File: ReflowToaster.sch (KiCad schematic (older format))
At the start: 3 parts, among them J2 USB-Micro-B, J3 USB-Micro-B, Q1 FDN340P

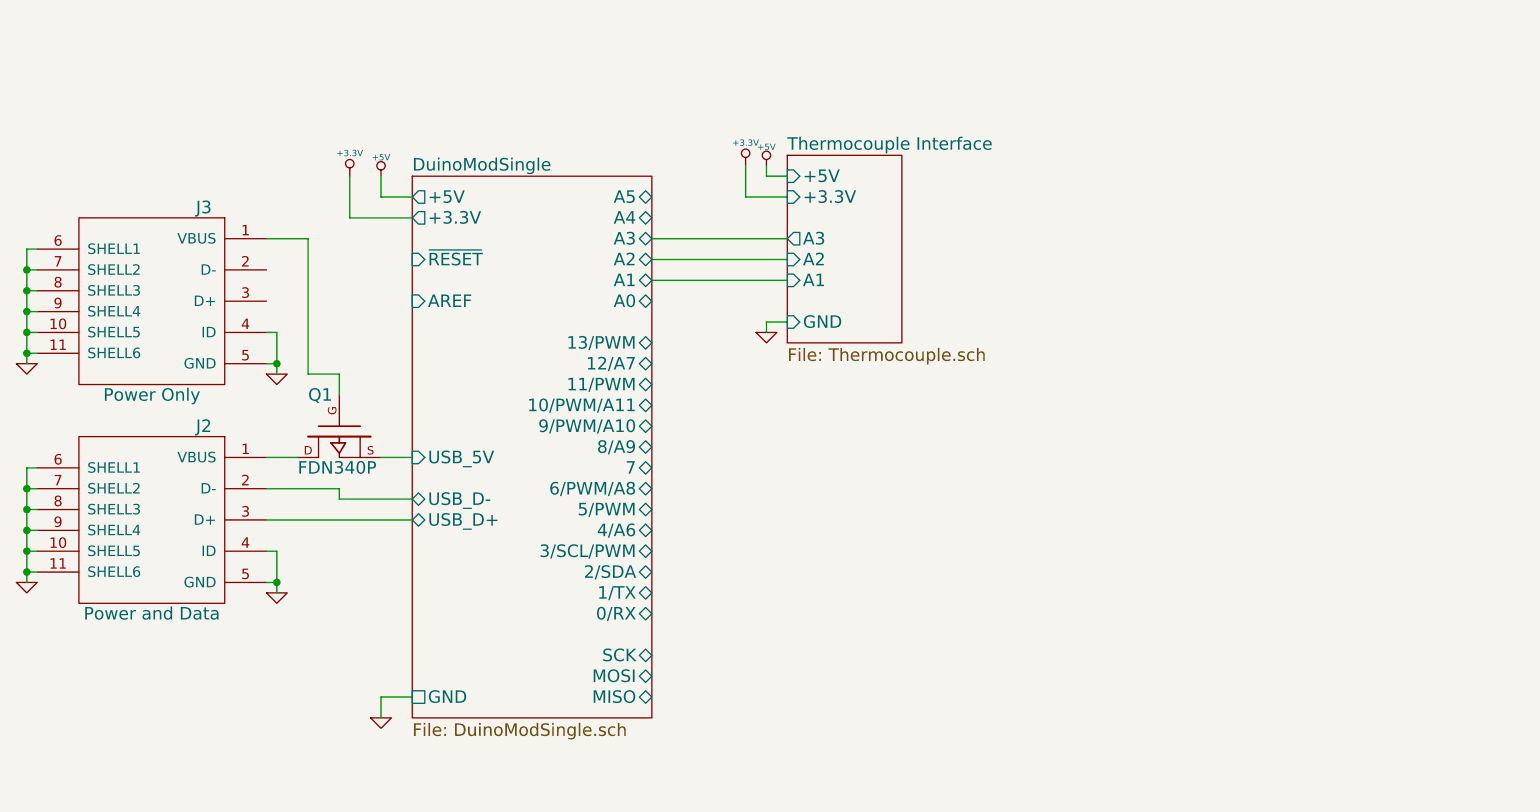
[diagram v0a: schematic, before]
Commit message: schematic complete
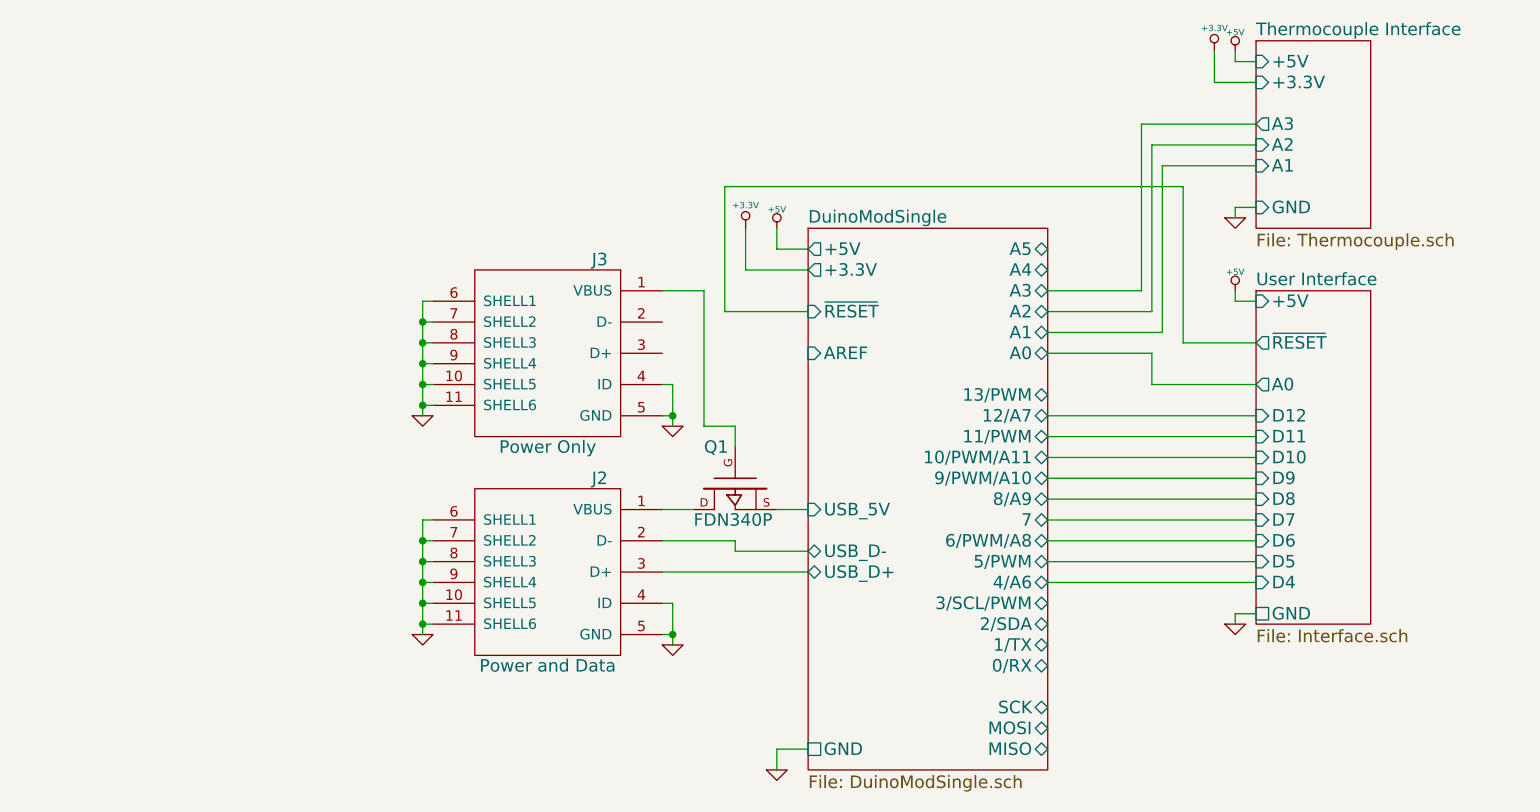
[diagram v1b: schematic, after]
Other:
- moved on the sheet: J2, J3, Q1
